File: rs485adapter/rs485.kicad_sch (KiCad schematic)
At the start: 15 parts, among them U1 MAX485E

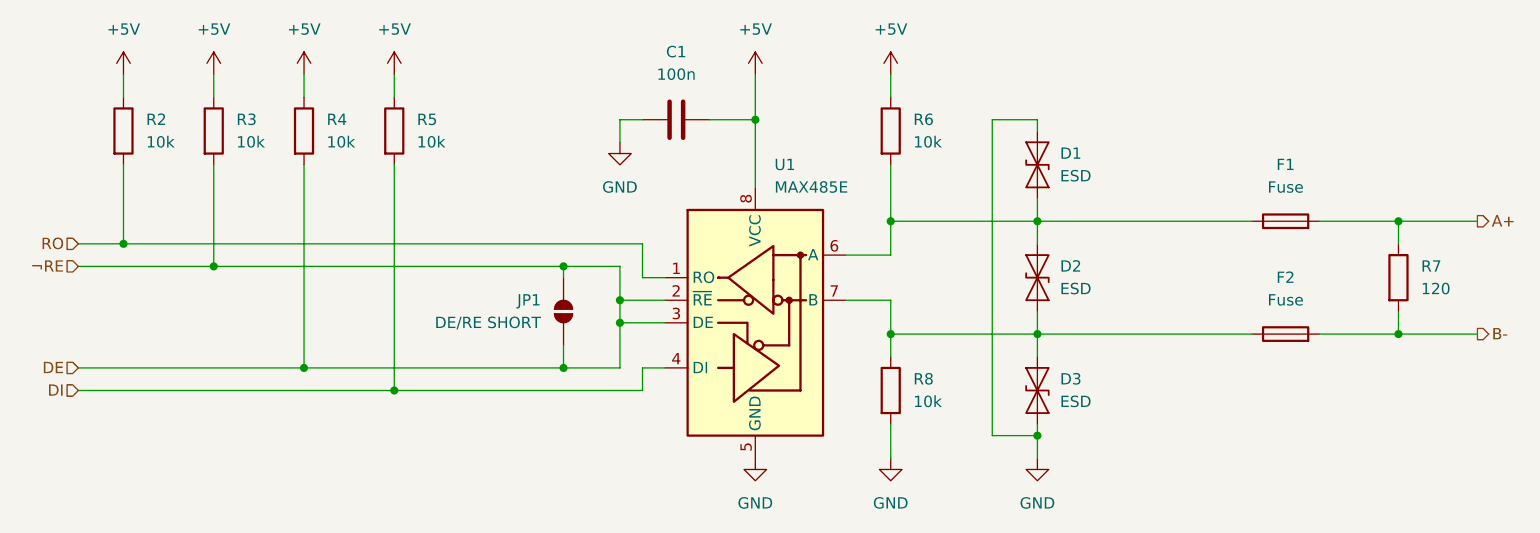
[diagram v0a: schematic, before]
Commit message: pushes
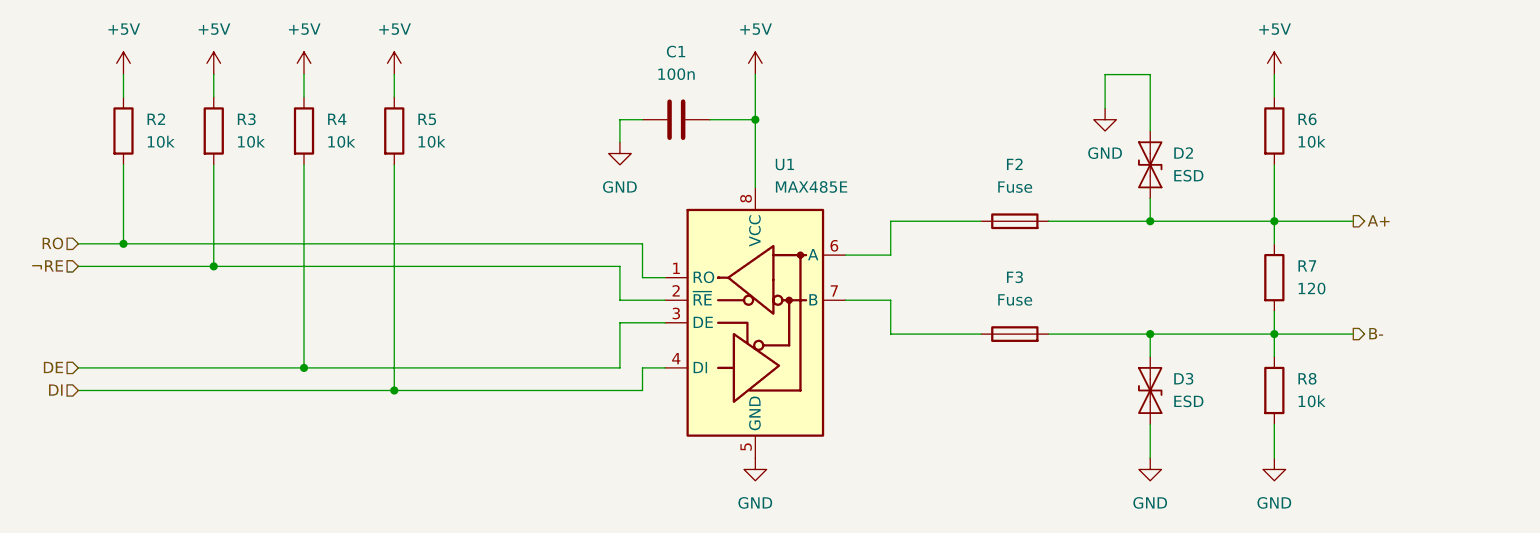
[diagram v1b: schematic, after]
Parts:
- removed D2: ESD, Diode_SMD:D_SMA, symbol Diode:ESD131-B1-W0201
- removed JP1: DE/RE SHORT, Jumper:SolderJumper-2_P1.3mm_Open_RoundedPad1.0x1.5mm, symbol Jumper:SolderJumper_2_Open
- C1: footprint Capacitor_SMD:C_0603_1608Metric -> Capacitor_SMD:C_0805_2012Metric
- R2, R3, R4, R5, R6, R7, R8: footprint Resistor_SMD:R_0603_1608Metric -> Resistor_SMD:R_0805_2012Metric
- renumbered D1 to D2, F1 to F2, F2 to F3
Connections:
- net A+: now also D2.2 (A2), R6.2
- net B-: now also D3.2 (A2), R8.1
- net DE: no longer R3.2, U1.2 (~{RE})
- net GND: now also D2.1 (A1); no longer D2.2 (A2)
- net at F2.1, U1.6 (A): no longer D2.1 (A1), R6.2
- net at F3.1, U1.7 (B): no longer D3.2 (A2), R8.1
- new net ¬RE: R3.2, U1.2 (~{RE})
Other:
- moved on the sheet: D2, D3, F2, F3, R7
